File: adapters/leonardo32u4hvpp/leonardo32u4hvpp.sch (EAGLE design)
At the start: 17 parts, among them J2 8x1F-H8.5, J3 8x1F-H8.5, J4 6x1F-H8.5, Y1 16MHz KX-7

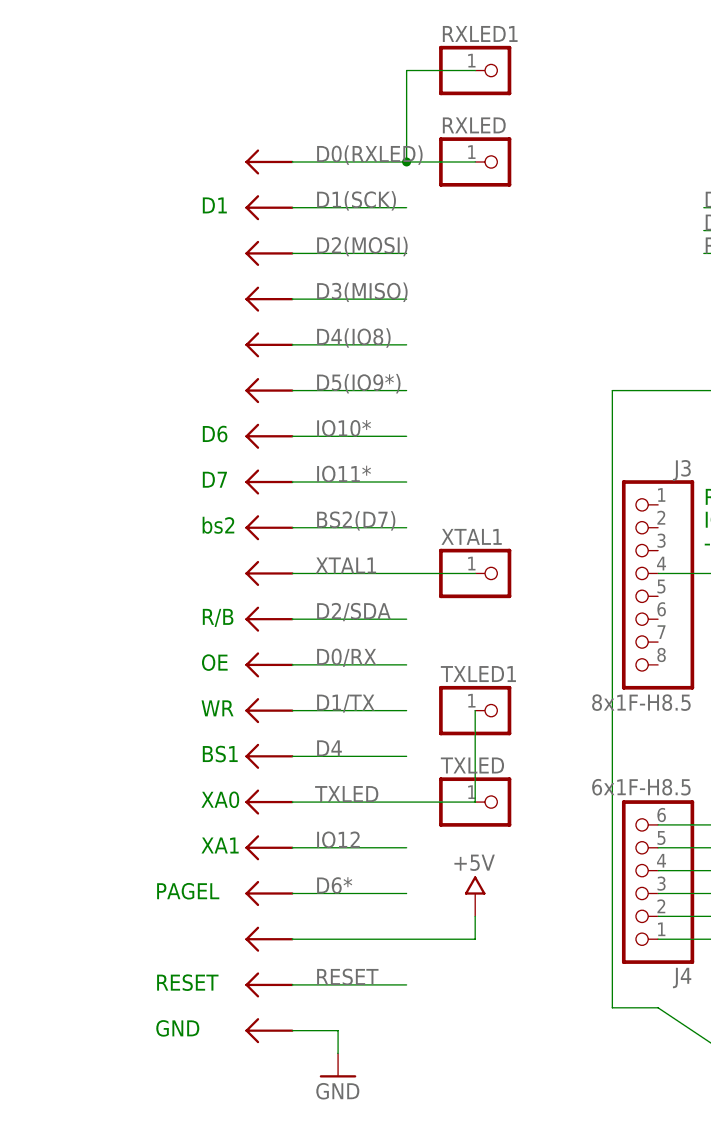
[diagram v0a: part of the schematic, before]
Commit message: t32u4
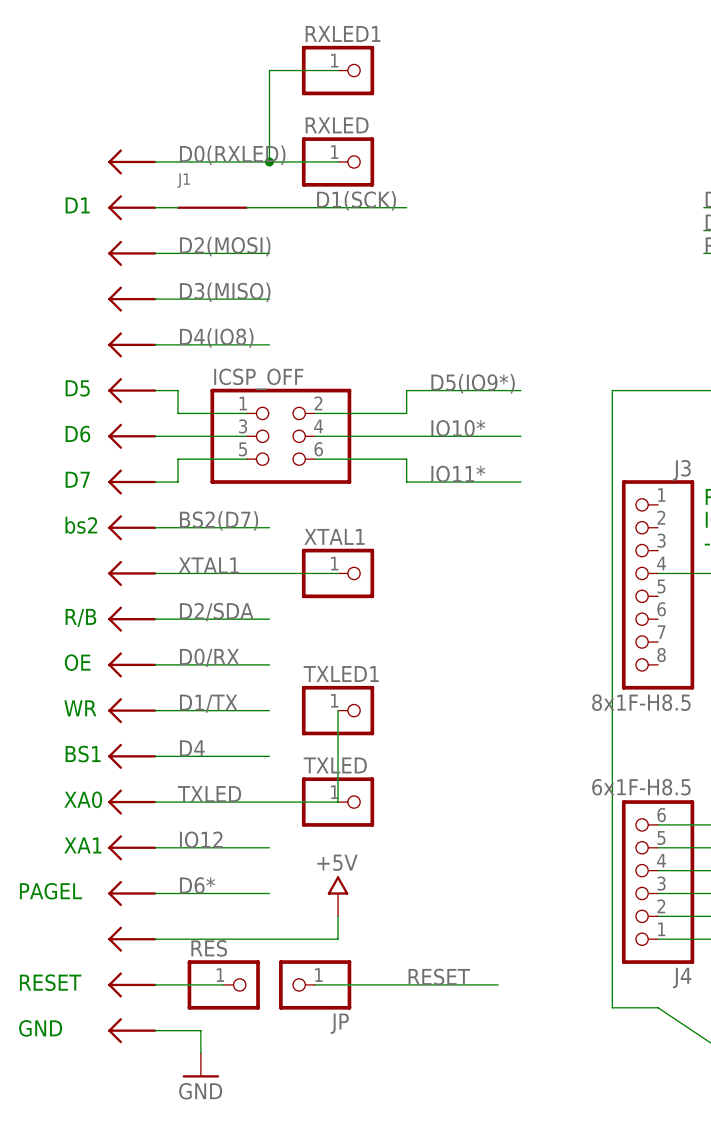
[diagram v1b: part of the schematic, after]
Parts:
- added ICSP_OFF: (no value), SmartPrj:PINHD-2X3
- added J1: J, detali_main:J
- added JP, RES: (no value), pinhead:PINHD-1X1
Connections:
- new net N$10: RES.1, U$2.RESET
- new net N$4: J1.P$2, U$2.D1
- new net N$5: ICSP_OFF.5, U$2.D7
- new net N$6: ICSP_OFF.3, U$2.D6
- new net N$8: ICSP_OFF.1, U$2.D5
- net D1(SCK): now also J1.P$1; no longer U$2.D1
- net D5(IO9*): now also ICSP_OFF.2; no longer U$2.D5
- net IO10*: now also ICSP_OFF.4; no longer U$2.D6
- net IO11*: now also ICSP_OFF.6; no longer U$2.D7
- net RESET: now also JP.1; no longer U$2.RESET
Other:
- note added: "D5"
- moved on the sheet: RXLED, RXLED1, TXLED, TXLED1, XTAL1
